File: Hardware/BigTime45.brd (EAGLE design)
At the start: 24.9 x 24.9 mm, 18 parts, among them J1 AVR_SPI_PRG_6TESTPOINTS-SM, U2 ATMEGA328P_TQFP, Y1 32.768kHz

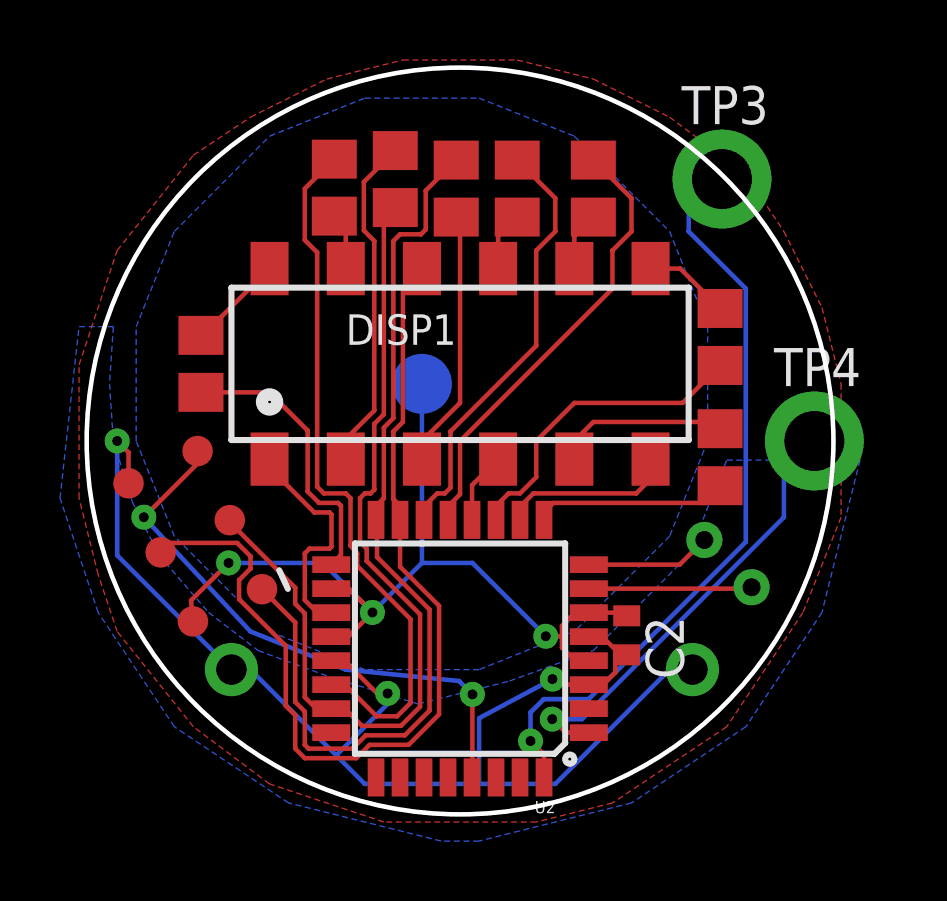
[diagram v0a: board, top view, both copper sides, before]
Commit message: tweak
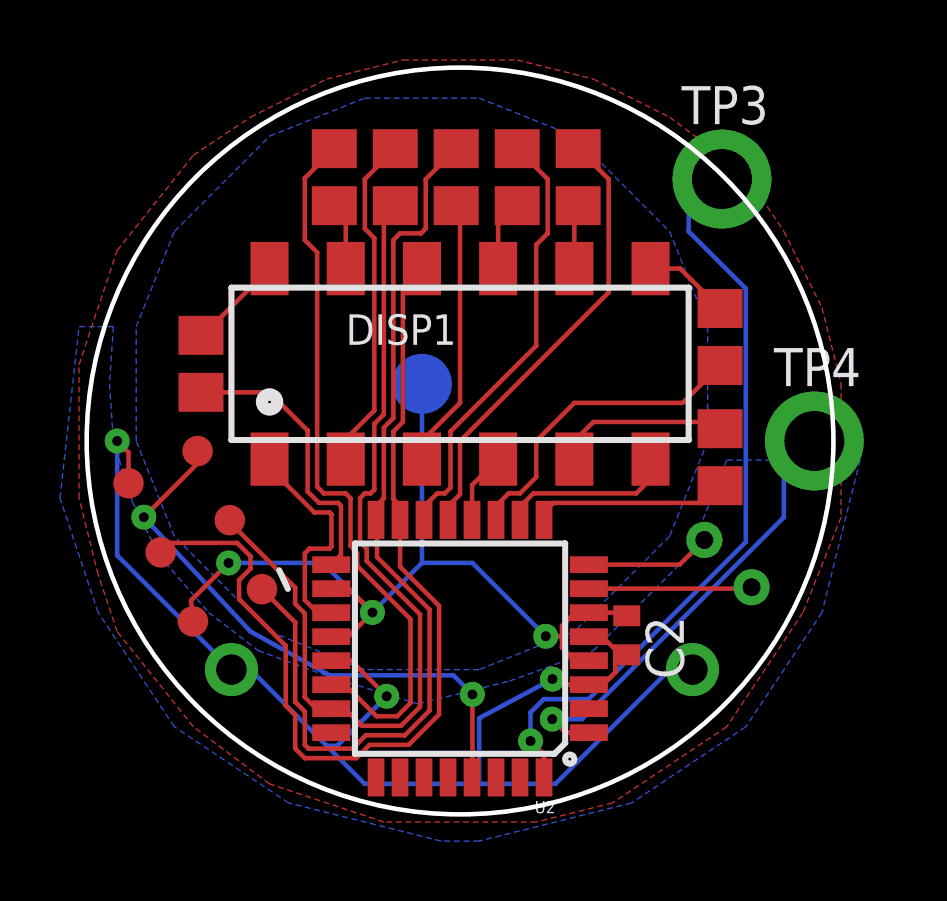
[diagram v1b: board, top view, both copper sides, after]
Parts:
- moved R5 0.63 mm to (18.5, 25.3)
- moved R4 0.38 mm to (14.5, 25.3)
- moved R7 0.38 mm to (16.5, 25.3)
- moved R3 0.35 mm to (10.4, 25.3)
- moved R6 0.06 mm to (12.4, 25.3)

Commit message: tweak
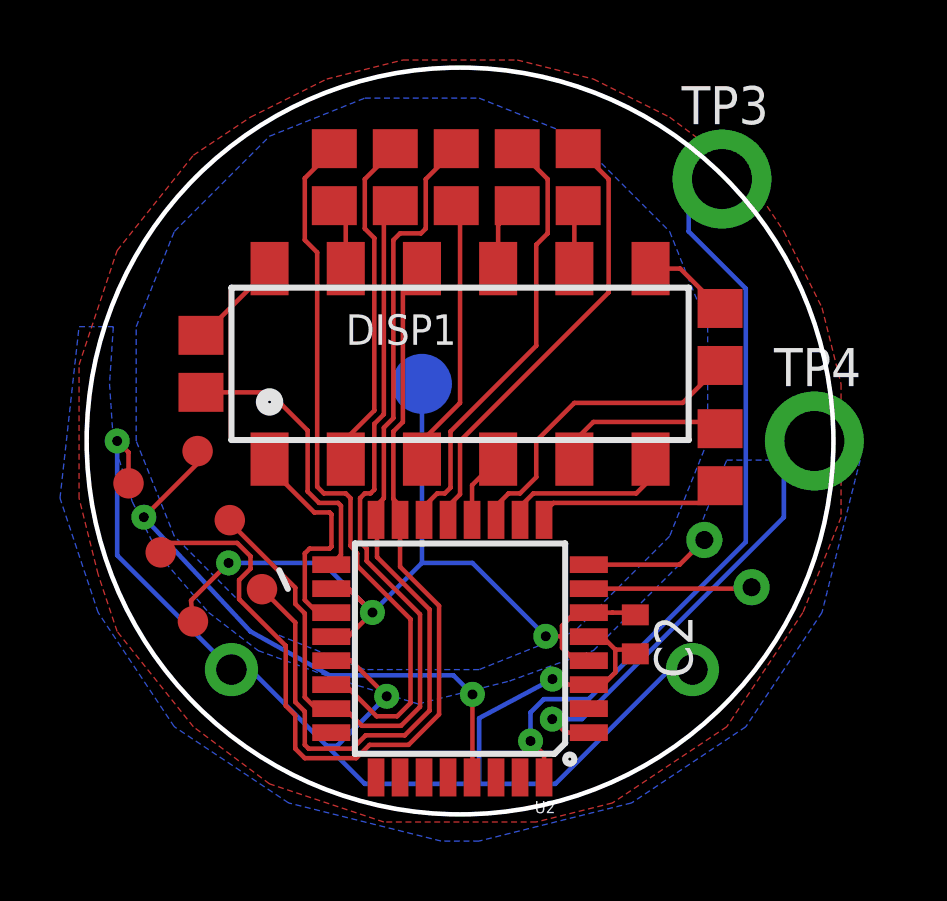
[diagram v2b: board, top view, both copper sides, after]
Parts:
- moved C2 0.29 mm to (20.4, 10.1)
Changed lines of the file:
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@@
 </autorouter>
 <elements>
-<element name="C2" library="resistor" package="C0402" value="100nF" x="20.16125" y="10.033" rot="R270"/>
+<element name="C2" library="resistor" package="C0402" value="100nF" x="20.447" y="10.06475" rot="R270"/>
 <element name="Y1" library="BigTime" package="TC26H" value="32.768kHz" x="22.63775" y="11.52525" smashed="yes" rot="MR225">
 <attribute name="NAME" x="20.213071875" y="11.076240625" size="1.27" layer="26" ratio="10" rot="MR315" display="off"/>
@@
 <wire x1="18.00225" y1="9.62025" x2="18.00225" y2="10.00125" width="0.1524" layer="1"/>
 <wire x1="18.00225" y1="10.00125" x2="18.00225" y2="10.3505" width="0.1524" layer="1"/>
-<wire x1="20.16125" y1="10.683" x2="20.432" y2="10.683" width="0.1524" layer="1"/>
+<wire x1="20.447" y1="10.71475" x2="20.432" y2="10.683" width="0.1524" layer="1"/>
 <wire x1="20.432" y1="10.683" x2="20.32" y2="10.795" width="0.1524" layer="1"/>
-<wire x1="18.8976" y1="10.7885" x2="20.05575" y2="10.7885" width="0.1524" layer="1"/>
-<wire x1="20.05575" y1="10.7885" x2="20.16125" y2="10.683" width="0.1524" layer="1"/>
+<wire x1="18.8976" y1="10.7885" x2="19.685" y2="10.7885" width="0.1524" layer="1"/>
+<wire x1="19.685" y1="10.7885" x2="20.05575" y2="10.7885" width="0.1524" layer="1"/>
 <wire x1="13.335" y1="12.446" x2="15.01775" y2="12.446" width="0.1524" layer="16"/>
 <wire x1="15.01775" y1="12.446" x2="17.4625" y2="10.00125" width="0.1524" layer="16"/>
@@
 <wire x1="6.88975" y1="12.446" x2="10.033" y2="12.446" width="0.1524" layer="16"/>
 <wire x1="10.033" y1="12.446" x2="11.684" y2="10.795" width="0.1524" layer="16"/>
+<wire x1="20.447" y1="10.71475" x2="20.37325" y2="10.7885" width="0.1524" layer="1"/>
+<wire x1="20.37325" y1="10.7885" x2="20.05575" y2="10.7885" width="0.1524" layer="1"/>
 </signal>
 <signal name="DIG1">
@@
 <wire x1="18.8976" y1="9.9885" x2="19.3485" y2="9.9885" width="0.1524" layer="1"/>
 <wire x1="19.3485" y1="9.9885" x2="19.78025" y2="9.55675" width="0.1524" layer="1"/>
-<wire x1="19.78025" y1="9.55675" x2="19.9875" y2="9.55675" width="0.1524" layer="1"/>
-<wire x1="19.9875" y1="9.55675" x2="20.16125" y2="9.383" width="0.1524" layer="1"/>
 <via x="17.68475" y="8.5725" extent="1-16" drill="0.3302"/>
 <wire x1="15.24" y1="5.08" x2="17.78" y2="5.08" width="0.1524" layer="16"/>
@@
 <wire x1="10.50925" y1="6.35" x2="10.16" y2="6.35" width="0.1524" layer="16"/>
 <wire x1="10.97275" y1="9.1885" x2="12.16025" y2="8.001" width="0.1524" layer="1"/>
+<wire x1="20.447" y1="9.41475" x2="20.305" y2="9.55675" width="0.1524" layer="1"/>
+<wire x1="20.305" y1="9.55675" x2="19.78025" y2="9.55675" width="0.1524" layer="1"/>
 </signal>
 <signal name="28">
